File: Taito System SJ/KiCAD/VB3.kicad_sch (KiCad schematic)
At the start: 29 parts, among them U1 74LS157, U13 74LS157, U14 74LS157, U15 74LS175, U19 74LS32, U2 74LS157, U27 74LS273, U28 74LS86, U29 74LS163, U33 74LS27, U39 74LS32, U4 74LS04, U40 74LS174, U41 RAM_5501, U42 74LS86, U43 74LS163, U5 74LS74, U54 74LS10, U55 74LS86, U56 74LS27, U57 74LS163, U6 74LS32, U69 RAM_5501, U7 74LS74, U70 74LS86, U71 74LS163, U72 74LS08

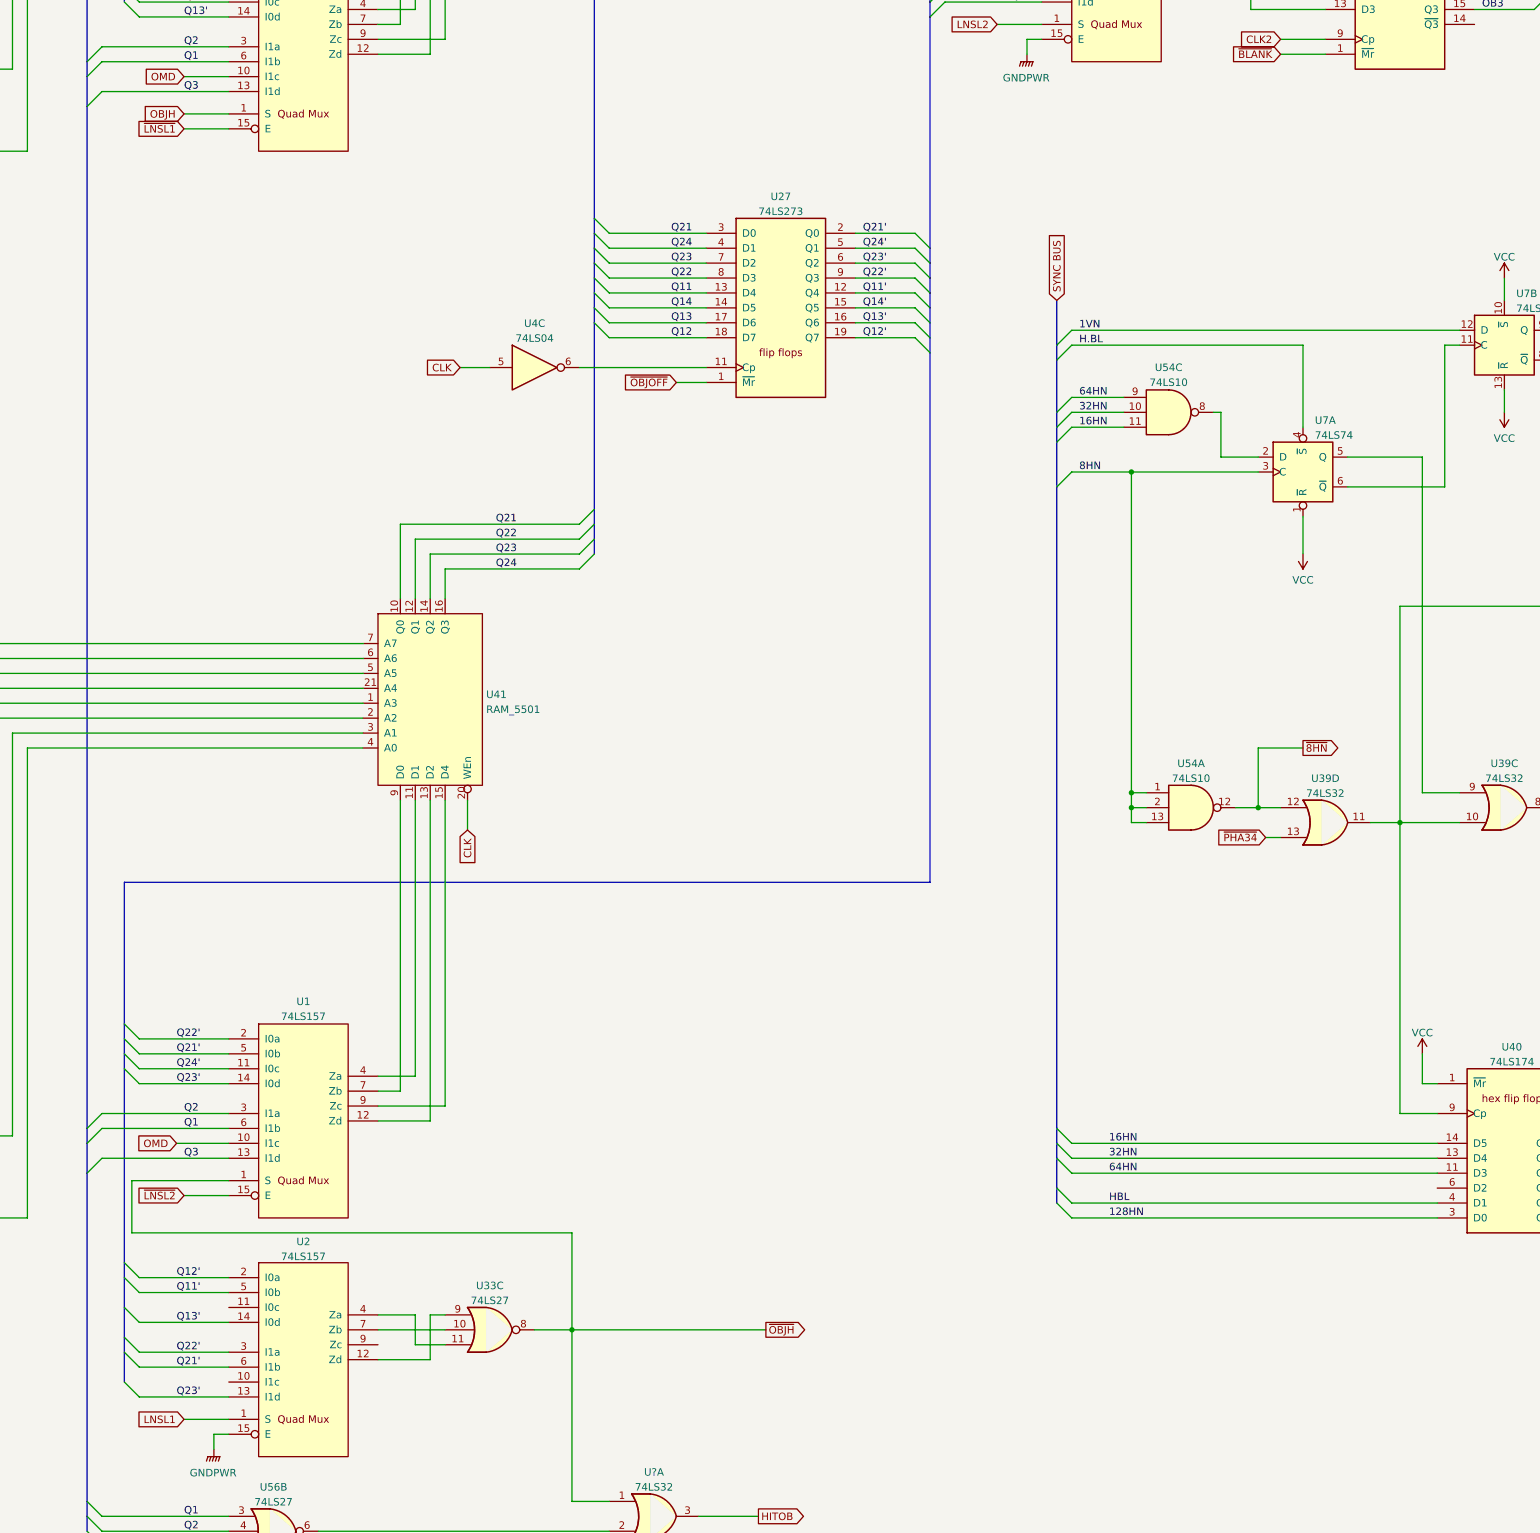
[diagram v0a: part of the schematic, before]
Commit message: Tidied up loose ends
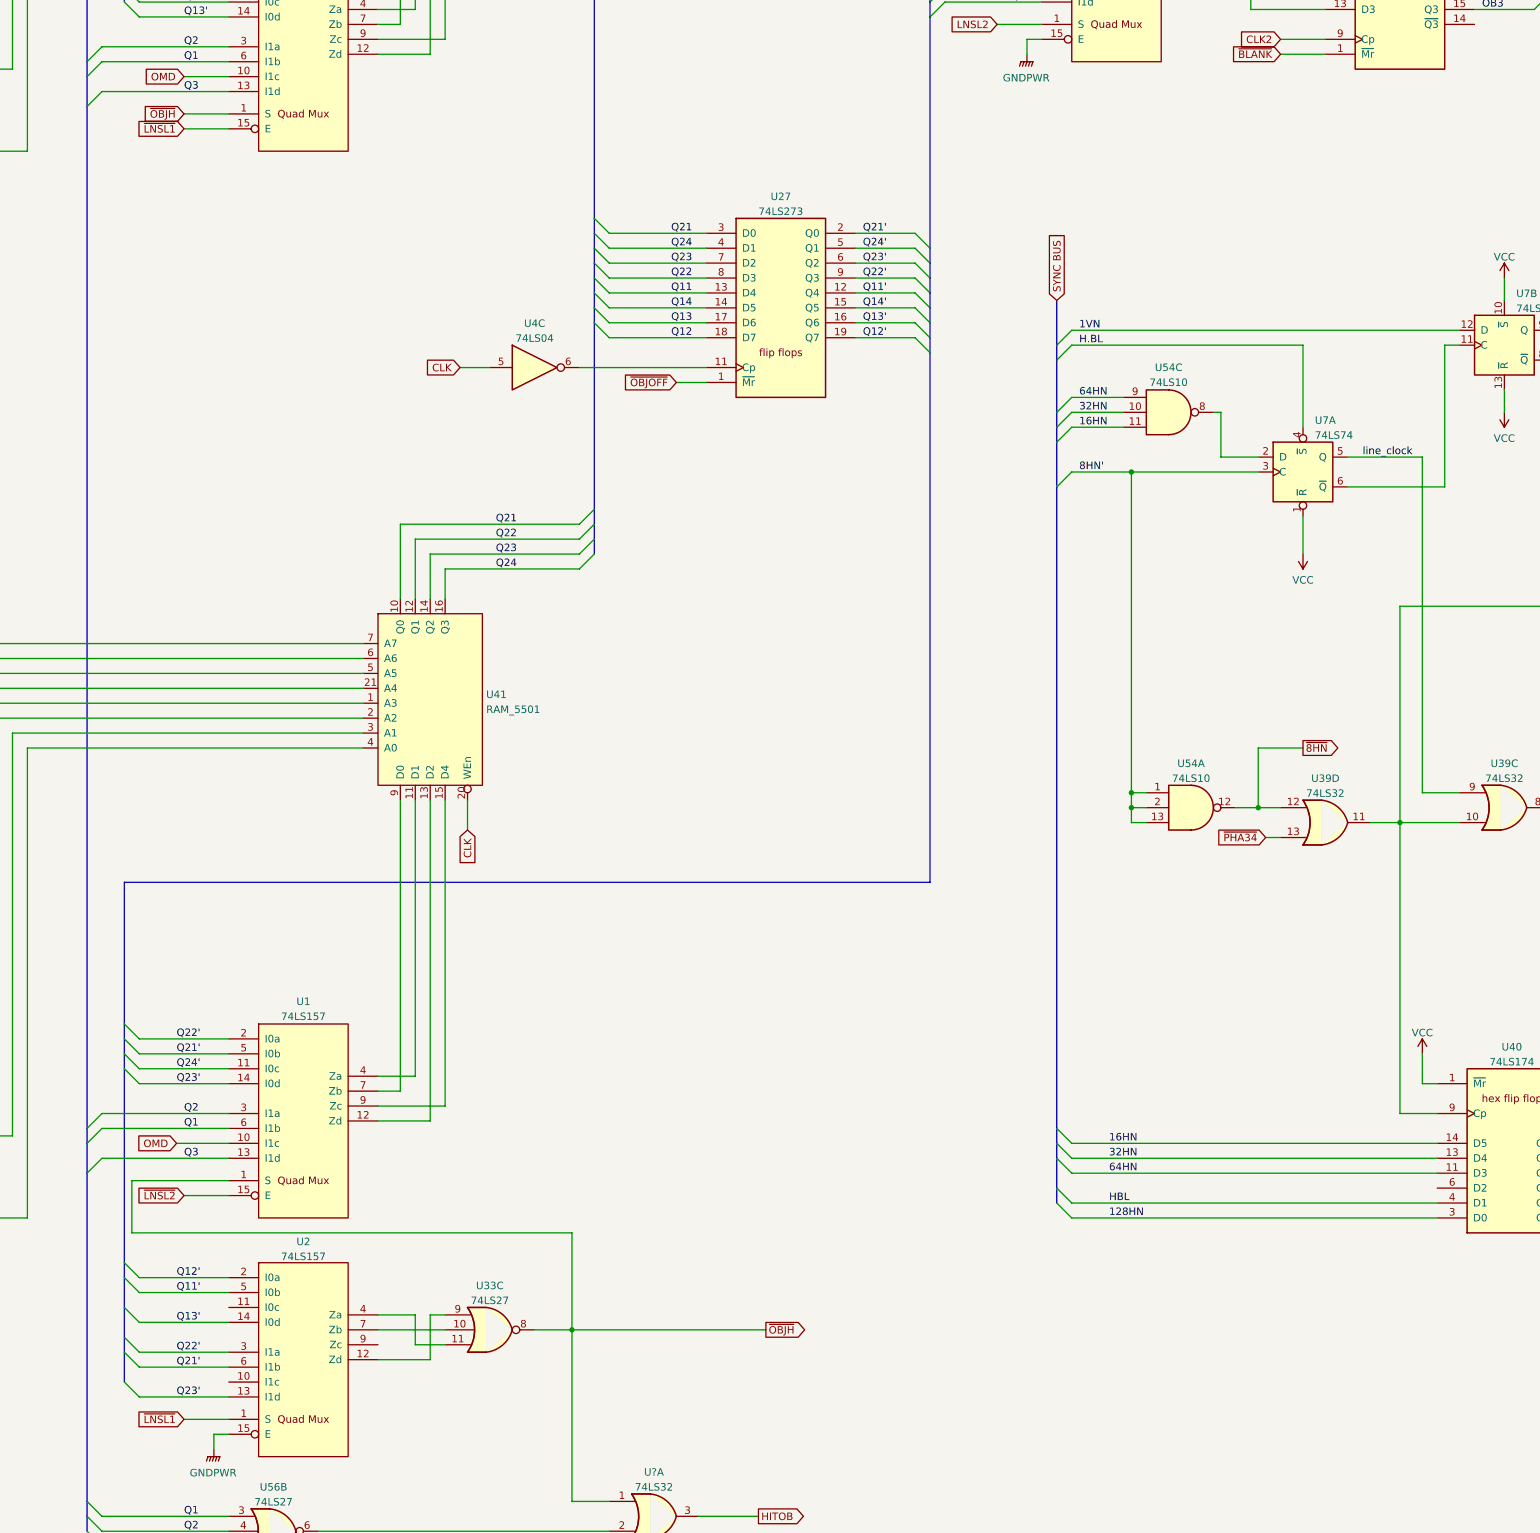
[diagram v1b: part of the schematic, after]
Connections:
- net LNSL1 is gone; now on net ~{LNSL1}: U2.1 (S)
- net OBJH is gone; now on net ~{OBJH}: U13.1 (S)
- net line_clock: now reaches U39.9, U7.5 (Q)
- net 8HN renamed 8HN'
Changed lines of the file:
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@@
     (effects (font (size 1.27 1.27)) (justify right bottom))
+  )
+  (label "line_clock" (at 394.97 210.82 0) (fields_autoplaced)
+    (effects (font (size 1.27 1.27)) (justify left bottom))
   )
   (label "Q22" (at 277.2376 180.34 0) (fields_autoplaced)
@@
     (effects (font (size 1.27 1.27)) (justify left bottom))
   )
-  (label "8HN" (at 346.71 213.36 0) (fields_autoplaced)
+  (label "8HN'" (at 346.71 213.36 0) (fields_autoplaced)
     (effects (font (size 1.27 1.27)) (justify left bottom))
   )
@@
     )
   )
-  (global_label "LNSL1" (shape input) (at 194.31 374.65 180) (fields_autoplaced)
-    (effects (font (size 1.27 1.27)) (justify right))
-    (property "Intersheetrefs" "${INTERSHEET_REFS}" (at 186.0912 374.5706 0)
+  (global_label "~{LNSL1}" (shape input) (at 194.31 374.65 180) (fields_autoplaced)
+    (effects (font (size 1.27 1.27)) (justify right))
+    (property "Intersheetrefs" "${INTERSHEET_REFS}" (at 185.5985 374.65 0)
       (effects (font (size 1.27 1.27)) (justify right) hide)
     )
@@
     )
   )
-  (global_label "OBJH" (shape input) (at 194.31 152.4 180) (fields_autoplaced)
+  (global_label "~{OBJH}" (shape input) (at 194.31 152.4 180) (fields_autoplaced)
     (effects (font (size 1.27 1.27)) (justify right))
     (property "Intersheetrefs" "${INTERSHEET_REFS}" (at 186.5056 152.4 0)

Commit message: Added MCU to Taito SJ Schematics
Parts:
- added U110: 74LS74, symbol jt74:74LS74
- added unit 5 of U4
- added unit 2 of U5
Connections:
- net CLK2: now also U110.11 (C), U110.3 (C)
- net H.INV: now also U110.1 (~{R}), U110.13 (~{R})
- net VCC: now also U110.10 (~{S}), U110.4 (~{S}), U5.10 (~{S}), U5.13 (~{R})
- net at U5.2 (D), U6.10, U6.5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: now also U5.12 (D)
- net at U19.6, U5.3 (C): now also U4.11
- new net: U110.2 (D), U5.9 (Q)
- new net: U4.10, U5.11 (C)
- new net: U110.12 (D), U5.8 (~{Q})
- new net ~{LNSL1X}: U110.5 (Q)
- new net ~{LNSL2X}: U110.9 (Q)
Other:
- note added: "ONLY ON FRONTLINE"
- moved on the sheet: U19B, U39C, U39D, U40, U54A, U54C, U5A, U6A, U6B, U6C, U6D, U7A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
